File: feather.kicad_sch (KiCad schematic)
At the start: 1 part

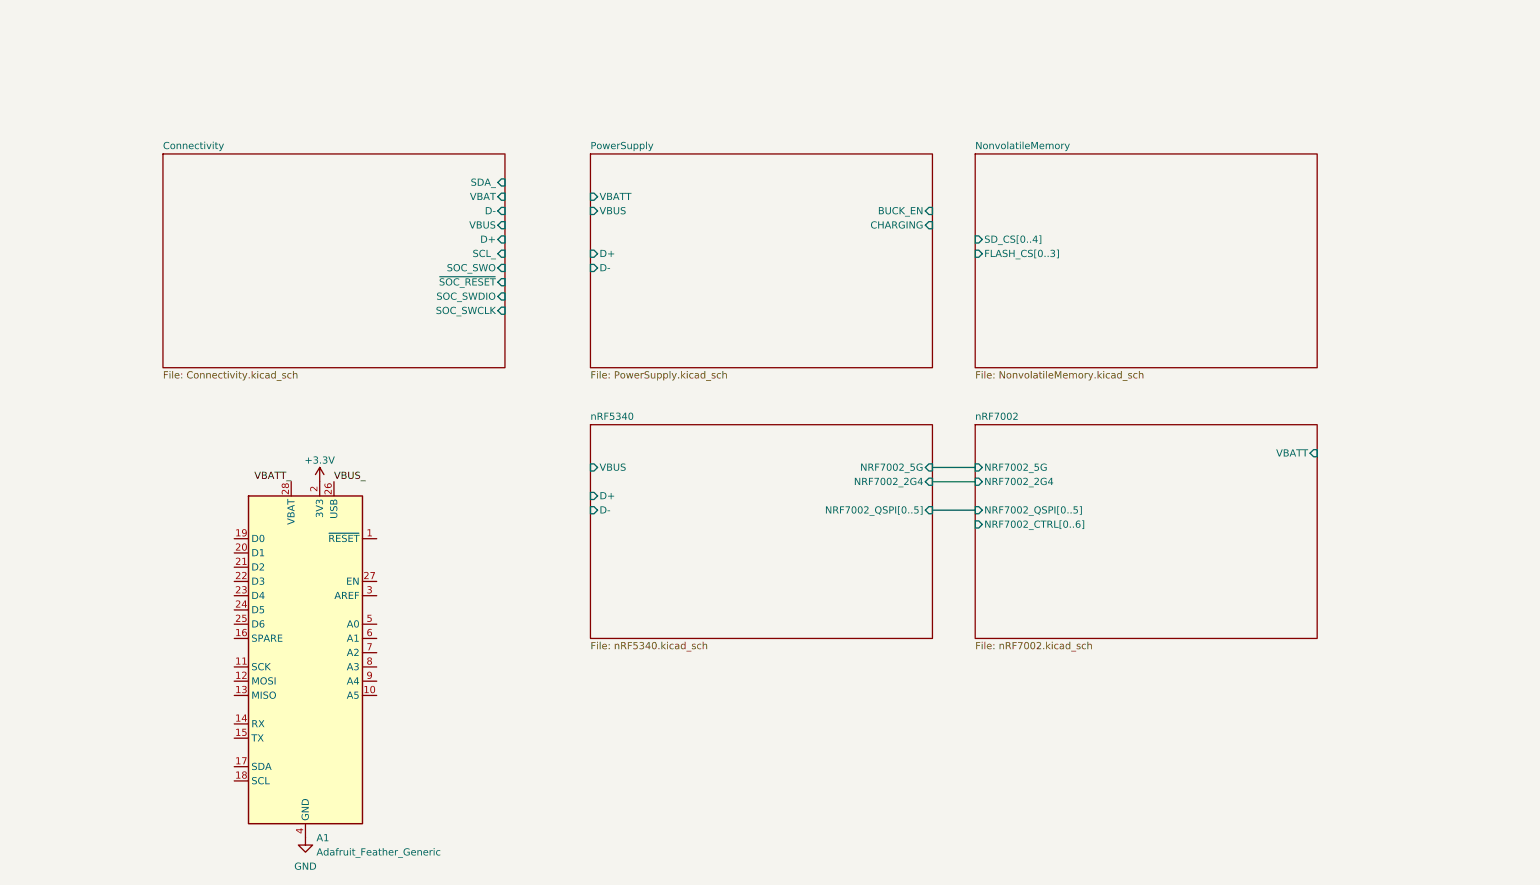
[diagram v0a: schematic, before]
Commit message: Schematic complete.
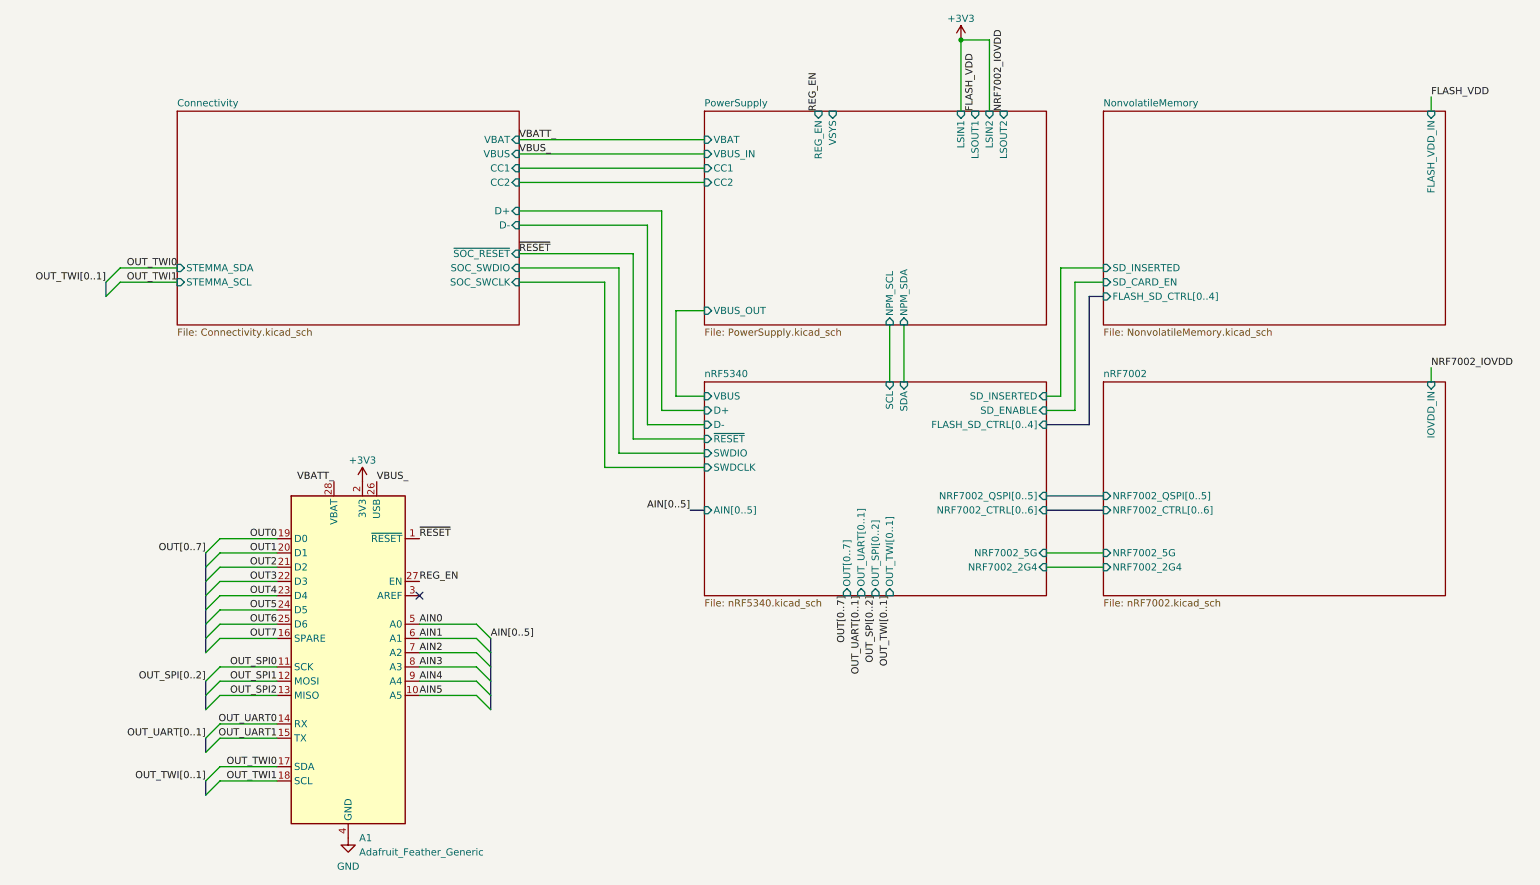
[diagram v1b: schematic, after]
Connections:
- net ~{RESET}: now reaches A1.1 (~{RESET})
- net AIN5: now reaches A1.10 (A5)
- net OUT_SPI0: now reaches A1.11 (SCK)
- net OUT_SPI1: now reaches A1.12 (MOSI)
- net OUT_SPI2: now reaches A1.13 (MISO)
- net OUT_UART0: now reaches A1.14 (RX)
- net OUT_UART1: now reaches A1.15 (TX)
- net OUT7: now reaches A1.16 (SPARE)
- net OUT_TWI0: now reaches A1.17 (SDA)
- net OUT_TWI1: now reaches A1.18 (SCL)
- net OUT0: now reaches A1.19 (D0)
- net OUT1: now reaches A1.20 (D1)
- net OUT2: now reaches A1.21 (D2)
- net OUT3: now reaches A1.22 (D3)
- net OUT4: now reaches A1.23 (D4)
- net OUT5: now reaches A1.24 (D5)
- net OUT6: now reaches A1.25 (D6)
- net REG_EN: now reaches A1.27 (EN)
- net AIN0: now reaches A1.5 (A0)
- net AIN1: now reaches A1.6 (A1)
- net AIN2: now reaches A1.7 (A2)
- net AIN3: now reaches A1.8 (A3)
- net AIN4: now reaches A1.9 (A4)
- net +3.3V renamed +3V3
- no-connect marks 0 -> 1
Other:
- sheet Connectivity ports: added CC1, CC2, STEMMA_SCL, STEMMA_SDA; removed SCL_, SDA_, SOC_SWO
- sheet NonvolatileMemory ports: added FLASH_SD_CTRL[0..4], FLASH_VDD_IN, SD_CARD_EN, SD_INSERTED; removed FLASH_CS[0..3], SD_CS[0..4]
- sheet PowerSupply ports: added CC1, CC2, LSIN1, LSIN2, LSOUT1, LSOUT2, NPM_SCL, NPM_SDA, REG_EN, VBAT, VBUS_IN, VBUS_OUT, VSYS; removed BUCK_EN, CHARGING, D+, D-, VBATT, VBUS
- sheet nRF5340 ports: added AIN[0..5], FLASH_SD_CTRL[0..4], NRF7002_CTRL[0..6], OUT[0..7], OUT_SPI[0..2], OUT_TWI[0..1], OUT_UART[0..1], SCL, SDA, SD_ENABLE, SD_INSERTED, SWDCLK, SWDIO, ~{RESET}; removed none
- sheet nRF7002 ports: added IOVDD_IN; removed VBATT
- moved on the sheet: A1
